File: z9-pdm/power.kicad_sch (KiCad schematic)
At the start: 26 parts, among them U22 TLV76733DRVx, U6 LMR14206

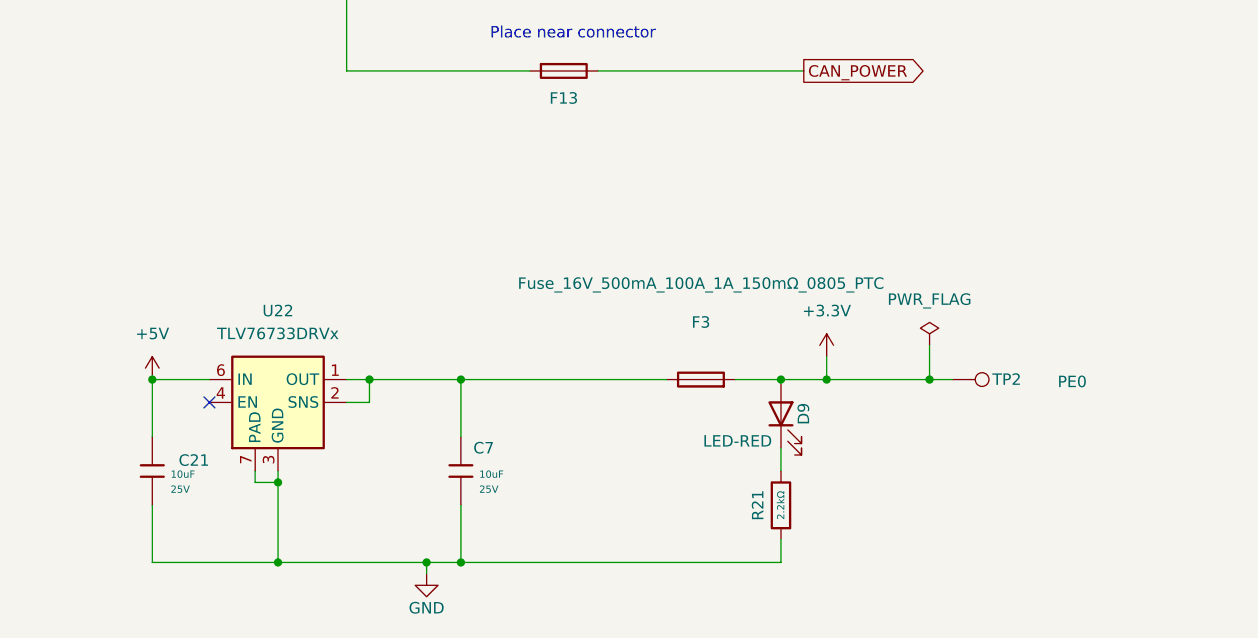
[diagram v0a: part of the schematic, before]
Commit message: x
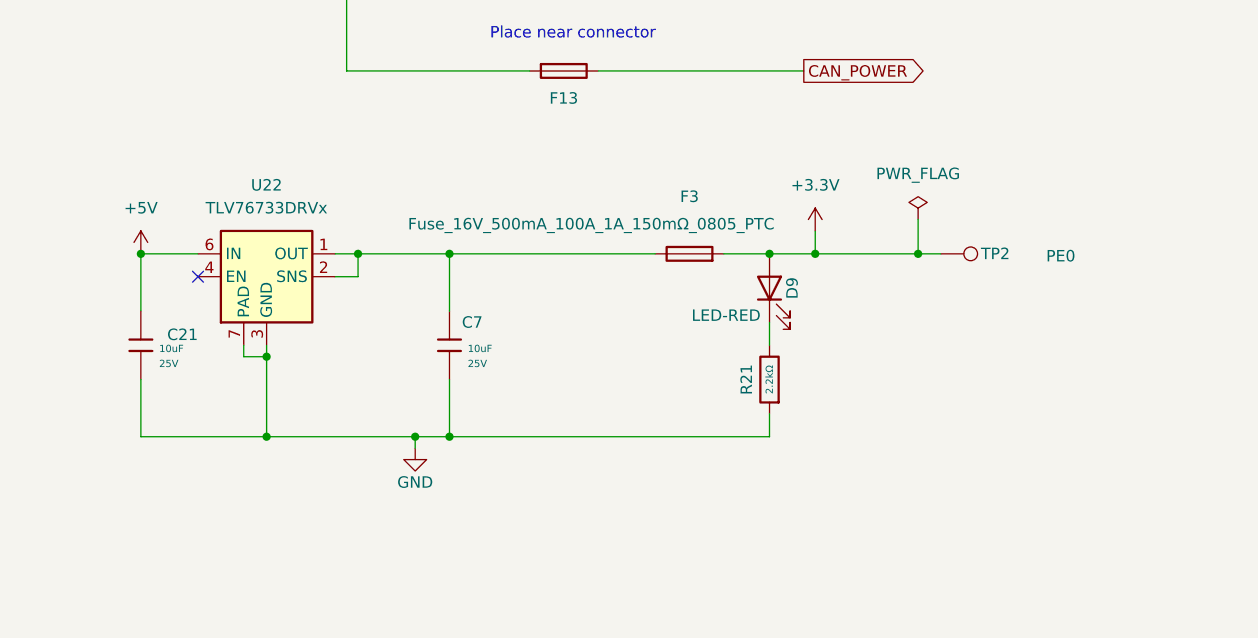
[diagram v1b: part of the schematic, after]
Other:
- moved on the sheet: C21, C7, D9, F3, R21, TP2, U22

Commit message: new fuse and ideal diode
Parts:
- removed D1: LED-RED, dnt:LED_0603_1608Metric - polarity, symbol dnt_global:LED-RED
- removed D2: B340, Diode_SMD:D_SMC, symbol Diode:B340
- removed D702: SM15T24A, PCM_Diode_SMD_AKL:D_SMC, symbol dnt_global:SM15T24A
- removed R4: 2.2kΩ, PCM_JLCPCB:R_0603, symbol PCM_JLCPCB-Resistors:0603,2.2kΩ
- added C18: 10uF, PCM_JLCPCB:C_0805, symbol PCM_JLCPCB-Capacitors:0805,10uF,(2)
- added C19, C27: 100nF, dnt:C_0603_1608Metric, symbol dnt_global:0603 100nF 50V X7R
- added C2, C4: 10uF, dnt:C_0603_1608Metric, symbol dnt_global:0603,10uF,_25V
- added C21: 22uF, PCM_JLCPCB:C_0805, symbol PCM_JLCPCB-Capacitors:0805,22uF
- added D21: Schotty V1P6-M3/H 60V 1A, Diode_SMD:D_MicroSMP_AK, symbol dnt_global:Diode - V1P6-M3/H 60V 1A Schotty
- added D22: LED-RED, dnt:LED_0603_1608Metric - polarity, symbol dnt_global:LED-RED
- added D3, D8: SMBJ18A, PCM_JLCPCB:D_SMB, symbol PCM_JLCPCB-Diodes:TVS-Uni,SMBJ18A
- added F4, F7, F8: Fuse_16V_500mA_100A_1A_150mΩ_PTC, Fuse:Fuse_0805_2012Metric, symbol dnt_global:Fuse_16V_500mA_100A_1A_150mΩ_0805_PTC_Resettable_Fuses_ROHS
- added L3: 3.3uH, Inductor_SMD:L_Sunlord_SWPA4030S, symbol dnt_global:L_Ferrite_-_Inductor_with_ferrite_core_-__2.4A_3.3uH_±20%_3.6A_SMD,4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
- added Q4: DMT6007LFG, PCM_Package_SON_AKL:Diodes_PowerDI3333-8, symbol PCM_Transistor_MOSFET_AKL:DMT6007LFG
- added R16: 56kΩ, PCM_JLCPCB:R_0603, symbol PCM_JLCPCB-Resistors:0603,56kΩ
- added R17: 10kΩ, PCM_JLCPCB:R_0603, symbol PCM_JLCPCB-Resistors:0603,10kΩ
- added R18: 2.2kΩ, PCM_JLCPCB:R_0603, symbol PCM_JLCPCB-Resistors:0603,2.2kΩ
- added R23, R26: 100kΩ, PCM_JLCPCB:R_0603, symbol dnt_global:0603,100kΩ
- added R25: 10kΩ, dnt:R_0603_1608Metric, symbol dnt_global:0603,10kΩ
- added R27, R28, R29: 15kΩ, PCM_JLCPCB:R_0402, symbol dnt_global:0402,15kΩ
- added TP5: PE0, TestPoint:TestPoint_Pad_D1.0mm, symbol dnt_global:TestPoint_Pad_D1.0mm
- added U1: TLV76733DRVx, Package_SON:WSON-6-1EP_2x2mm_P0.65mm_EP1x1.6mm_ThermalVias, symbol Regulator_Linear:TLV76733DRVx
- added U7: LMR14206, Package_TO_SOT_SMD:SOT-23-6, symbol Regulator_Switching:LMR14206
- added U8: LM74700, Package_TO_SOT_SMD:SOT-23-6, symbol Power_Management:LM74700
- added U9: VN9016AJTR, POWERSSO16_3p9X4p9X0p5_STM, symbol dnt_global:VN9016AJTR
- C3: renamed from C21; footprint PCM_JLCPCB:C_0603 -> dnt:C_0603_1608Metric; symbol PCM_JLCPCB-Capacitors:0603,10uF,(2) -> dnt_global:0603,10uF,_25V
- C5: renamed from C7; footprint PCM_JLCPCB:C_0603 -> dnt:C_0603_1608Metric; symbol PCM_JLCPCB-Capacitors:0603,10uF,(2) -> dnt_global:0603,10uF,_25V
- C7: renamed from C18; footprint PCM_JLCPCB:C_0603 -> dnt:C_0603_1608Metric; symbol PCM_JLCPCB-Capacitors:0603,100nF -> dnt_global:0603 100nF 50V X7R
- F2: renamed from F13; value Fuse_16V_500mA_100A_1A_150mΩ_0805_PTC_Resettable_Fuses_ROHS -> Fuse_16V_500mA_100A_1A_150mΩ_PTC
- F3: value Fuse_16V_500mA_100A_1A_150mΩ_0805_PTC -> Fuse_16V_500mA_100A_1A_150mΩ_PTC
- F5: renamed from F1; value Fuse_16V_500mA_100A_1A_150mΩ_0805_PTC_Resettable_Fuses_ROHS -> Fuse_16V_500mA_100A_1A_150mΩ_PTC
- F6: renamed from F2; value Fuse_16V_500mA_100A_1A_150mΩ_0805_PTC_Resettable_Fuses_ROHS -> Fuse_16V_500mA_100A_1A_150mΩ_PTC
- TP2: now left out of the parts list
- TP3: renamed from TP1; now left out of the parts list
- renumbered C19 to C10, C3 to C6, D13 to D12, D8 to D19, D3 to D2, L1 to L2, R20 to R10, R21 to R4, R19 to R8, R18 to R9, U22 to U2
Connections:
- net +12V_VIPOWER: now also F7.1, U9.13 (OUTPUT0), U9.14 (OUTPUT0), U9.15 (OUTPUT0), U9.16 (OUTPUT0)
- net +BATT: now also C27.1, Q4.5 (D), R23.1, U8.6 (ANODE)
- net GND: now also C18.2, C2.2, C21.2, C4.2, D21.2 (A), D3.2, D8.2, R17.1, R18.1, U1.3 (GND), U1.5 (GND), U1.7 (PAD), U7.2 (GND), U8.2 (GND), U9.4 (GND)
- net +12V: no longer names the net of C6.1, F5.2, U6.4 (~{SHDN}), U6.5 (VIN)
- net +12V: now also D3.1
- new net: C4.1, F4.1, U1.1 (OUT), U1.2 (SNS)
- new net: D22.1 (K), R18.2
- new net: C21.1, F8.1, L3.2, R16.1
- new net: R16.2, R17.2, U7.3 (FB)
- new net: R27.2, U9.1 (INPUT0)
- new net: C18.1, D8.1, F7.2, U7.5 (VIN)
- new net: Q4.4 (G), R25.1
- new net: R25.2, R26.2, U8.5 (GATE)
- new net: Q4.1 (S), Q4.2 (S), Q4.3 (S), R26.1, U8.4 (CATHODE), U9.17 (EPAD)
- new net: C19.1, U7.1 (CB)
- new net: C19.2, D21.1 (K), L3.1, U7.6 (SW)
- new net: R29.2, U9.2 (*FAULTRST)
- new net: R28.2, U9.7 (CS)
- new net: R23.2, U8.3 (EN)
- new net: C27.2, U8.1 (VCAP)
- new net +3.3VA: F4.2
- new net +5VA: C2.1, D22.2 (A), F8.2, TP5.1, U1.6 (IN)
- new net 5VA_ENABLE: U7.4 (~{SHDN})
- no-connect marks 1 -> 2
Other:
- moved on the sheet: C10, C3, C5, C6, C7, D12, D19, D2, D9, F2, F3, F5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
